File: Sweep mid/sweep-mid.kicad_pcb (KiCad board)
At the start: 2 copper layers, 229.5 x 95.2 mm, 62 parts, among them J1 AudioJack4dpb, J2 AudioJack4dpb, SW10 SW_Push, SW11 SW_Push, SW11_r1 SW_Push, SW12 SW_Push, SW12_r1 SW_Push, SW13_r1 SW_Push, SW14 SW_Push, SW15 SW_Push, SW15_r1 SW_Push, SW16 SW_Push, SW16_r1 SW_Push, SW17 SW_Push, SW17_r1 SW_Push, SW18 SW_Push, SW18_r1 SW_Push, SW2 SW_Push, SW2 SW_SPDT, SW20 SW_Push, SW20_r1 SW_Push, SW21 SW_Push, SW21_r1 SW_Push, SW2_r1 SW_Push, SW3 SW_Push, SW3_r1 SW_Push, SW4 SW_Push, SW4_r1 SW_Push, SW5 SW_Push, SW5_r1 SW_Push, SW6 SW_Push, SW6_r1 SW_Push, SW7_r1 SW_Push, SW8 SW_Push, SW8_r1 SW_Push, SW9 SW_Push, SW9_r1 SW_Push, U1 ProMicro-kbd, U2 ProMicro-kbd

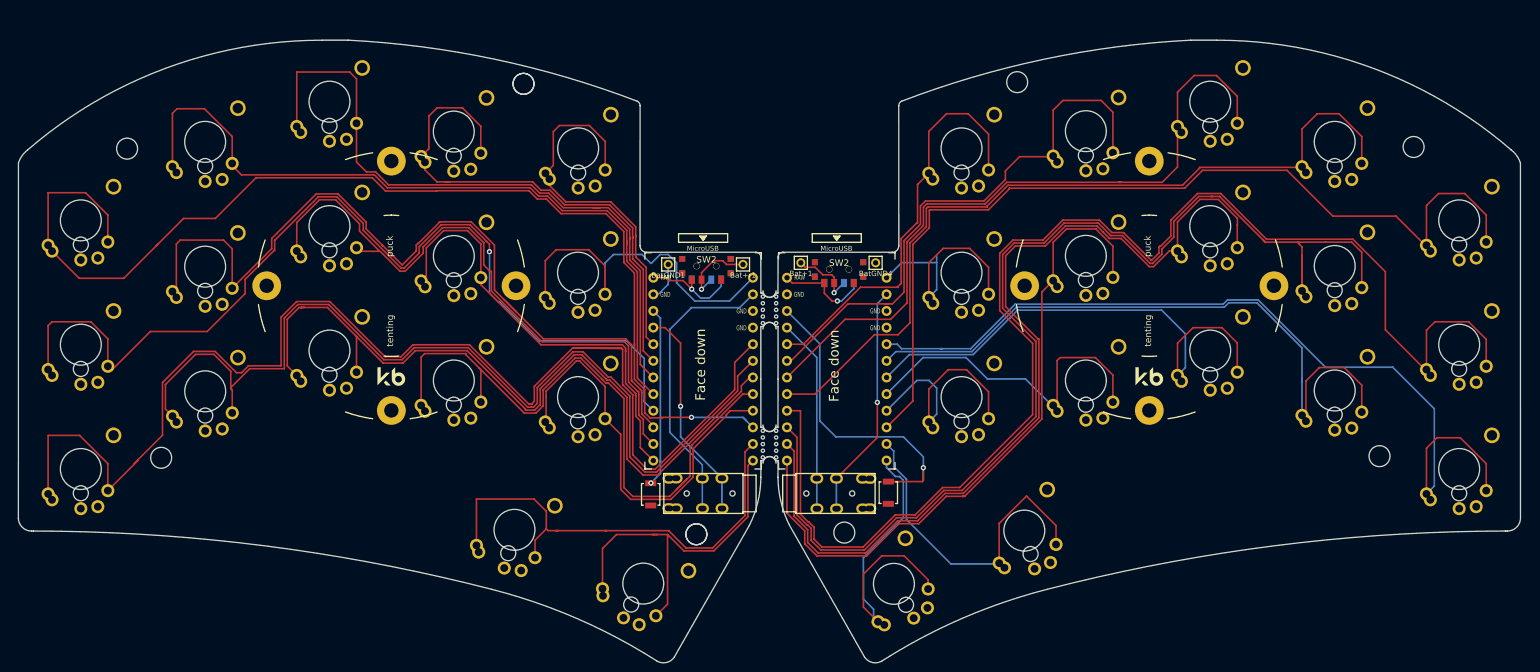
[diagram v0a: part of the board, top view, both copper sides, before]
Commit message: simplify footprint
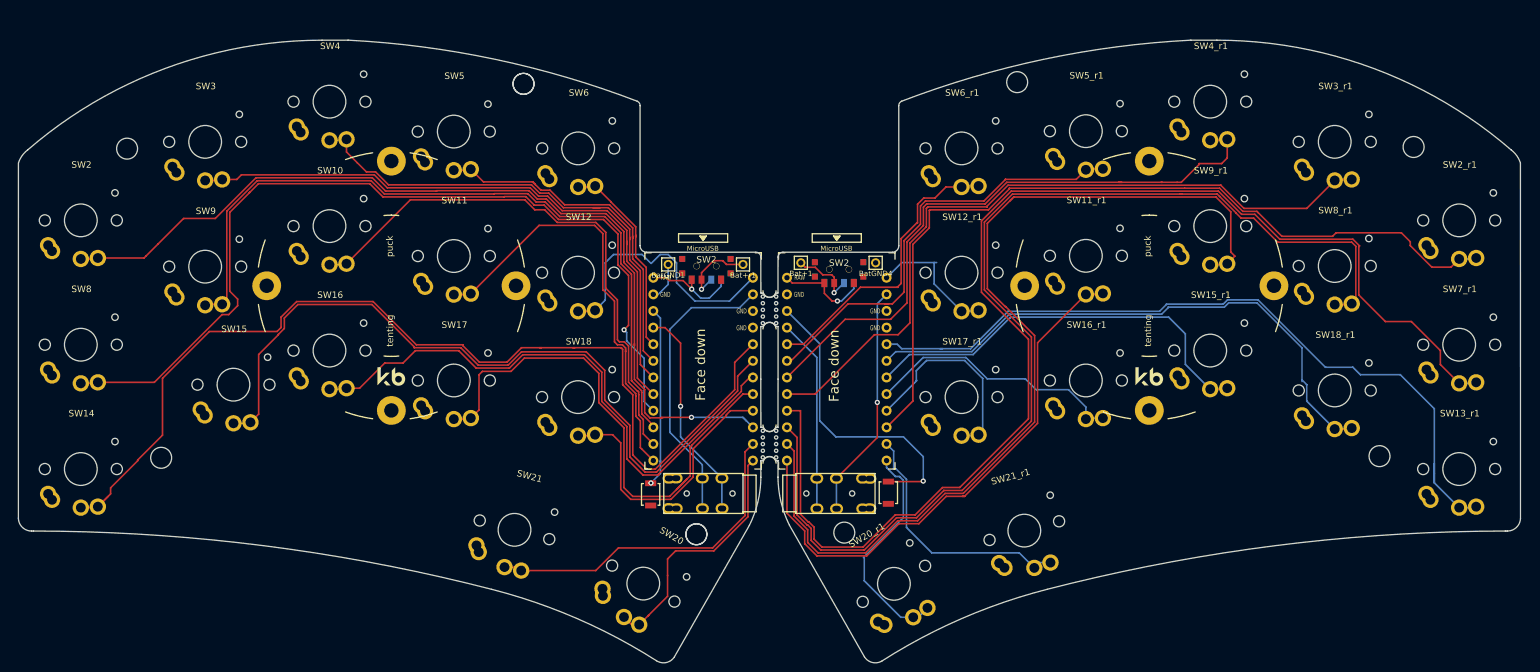
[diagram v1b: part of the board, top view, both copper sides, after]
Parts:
- SW10, SW11, SW11_r1, SW12, SW12_r1, SW13_r1, SW14, SW15, SW15_r1, SW16, SW16_r1, SW17, SW17_r1, SW18, SW18_r1, SW2, SW20, SW20_r1, SW21, SW21_r1, SW2_r1, SW3, SW3_r1, SW4, SW4_r1, SW5, SW5_r1, SW6, SW6_r1, SW7_r1, SW8, SW8_r1, SW9, SW9_r1: footprint mid:MXMountLP-1U -> sadik:gateron-ks27-choc-v1
- moved SW15 4.44 mm to (68.3, 102.1)
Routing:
- net Switch11: track 194.9 -> 156.7 mm
- net Switch1: track 170.7 -> 139.2 mm
- net Switch13: track 120.1 -> 89.0 mm
- net Switch12: track 148.7 -> 119.4 mm
- net Switch5: track 59.0 -> 30.8 mm
- net Switch4: track 80.8 -> 53.6 mm
- net Switch3: track 103.2 -> 78.3 mm
- net Switch14: track 102.0 -> 80.8 mm
- net Switch16: track 72.0 -> 51.9 mm
- net Switch15: track 63.1 -> 43.3 mm
- net Switch2: track 114.7 -> 95.5 mm
- net Switch9_r: track 103.2 -> 84.3 mm
- net Switch5_r: track 63.3 -> 45.1 mm
- net Switch4_r: track 84.8 -> 67.3 mm
- net Switch17_r: track 51.8 -> 35.0 mm
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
